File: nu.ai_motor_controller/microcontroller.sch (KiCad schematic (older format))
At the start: 31 parts

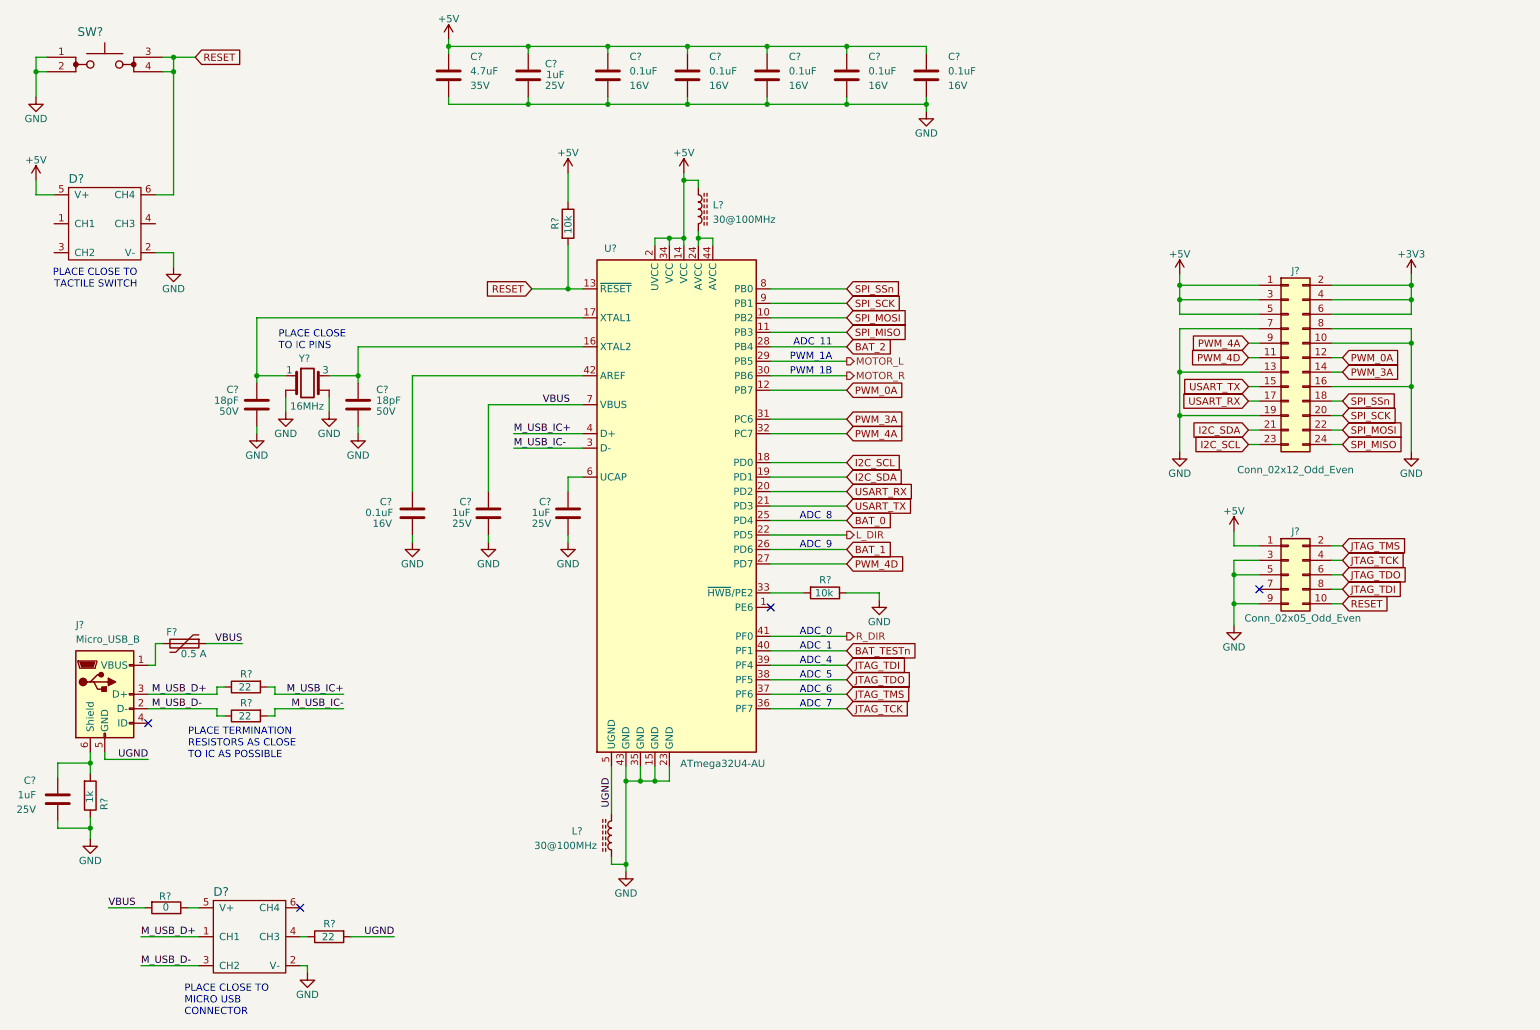
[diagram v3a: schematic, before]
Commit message: automated commit
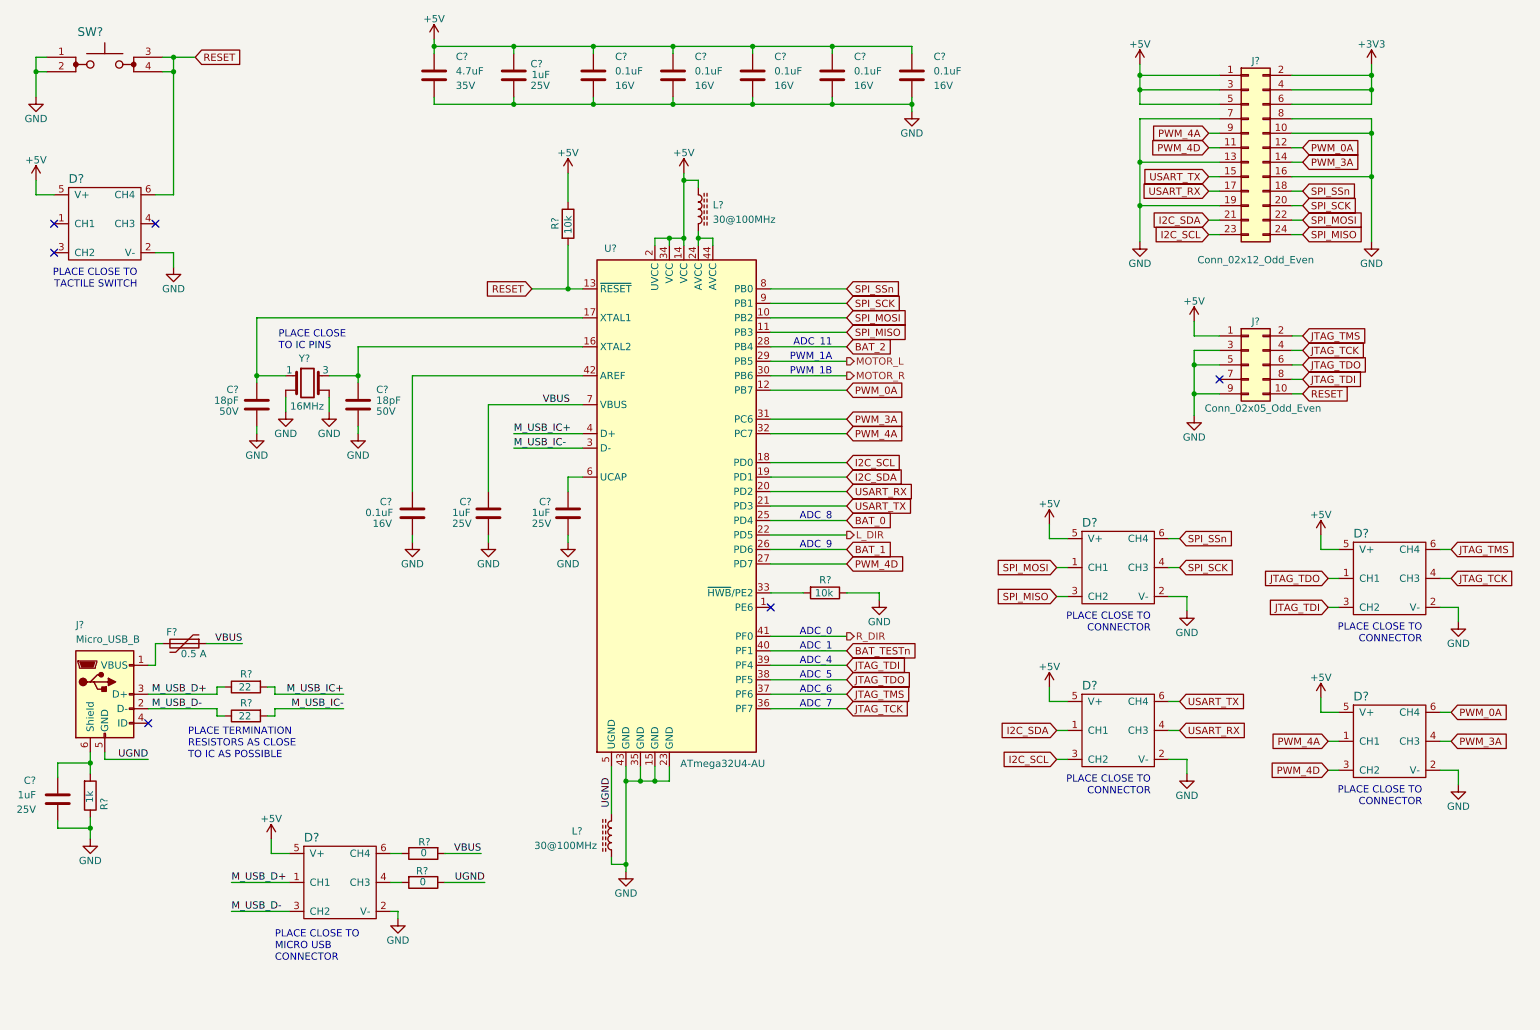
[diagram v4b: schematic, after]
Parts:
- removed R?: RMCF0603FT22R0, 0603, symbol custom:RMCF0603FT22R0
- added D? (x4): CM1293A-04SO, SOT-457, symbol custom:CM1293A-04SO
- added R?: RC0603JR-070RL, Resistor_SMD:R_0603_1608Metric, symbol custom:RC0603JR-070RL
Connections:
- net +5V: now also D?.5 (V+), D?.5 (V+), D?.5 (V+), D?.5 (V+), D?.5 (V+)
- net GND: now also D?.2 (V-), D?.2 (V-), D?.2 (V-), D?.2 (V-)
- net I2C_SCL: now also D?.3 (CH2)
- net I2C_SDA: now also D?.1 (CH1)
- net JTAG_TCK: now also D?.4 (CH3)
- net JTAG_TDI: now also D?.3 (CH2)
- net JTAG_TDO: now also D?.1 (CH1)
- net JTAG_TMS: now also D?.6 (CH4)
- net PWM_0A: now also D?.6 (CH4)
- net PWM_3A: now also D?.4 (CH3)
- net PWM_4A: now also D?.1 (CH1)
- net PWM_4D: now also D?.3 (CH2)
- net SPI_MISO: now also D?.3 (CH2)
- net SPI_MOSI: now also D?.1 (CH1)
- net SPI_SCK: now also D?.4 (CH3)
- net SPI_SSn: now also D?.6 (CH4)
- net UGND: now also R?.1
- net USART_RX: now also D?.4 (CH3)
- net USART_TX: now also D?.6 (CH4)
- net at D?.4 (CH3): now also R?.2
- net at R?.1: now also D?.6 (CH4); no longer D?.5 (V+)
- no-connect marks 4 -> 6
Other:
- note added: "PLACE CLOSE TO\nCONNECTOR"
- moved on the sheet: C?, D?, J?, R?

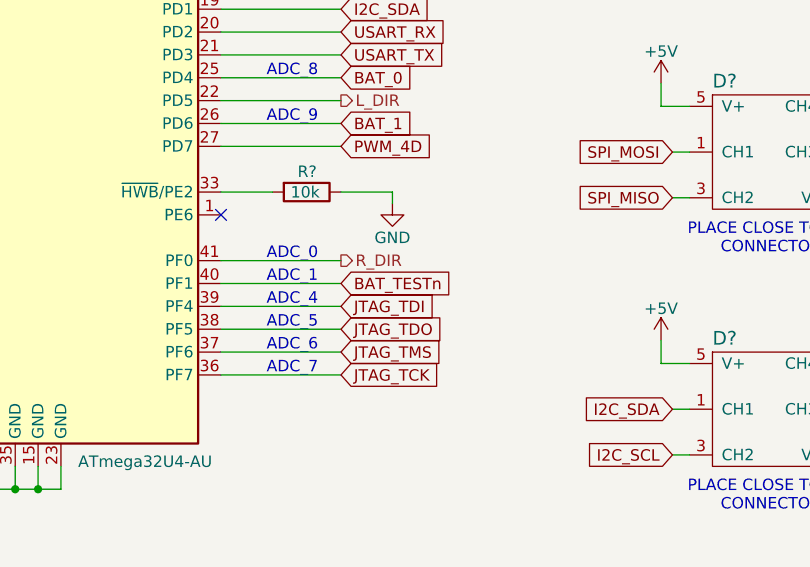
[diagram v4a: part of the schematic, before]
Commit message: automated commit
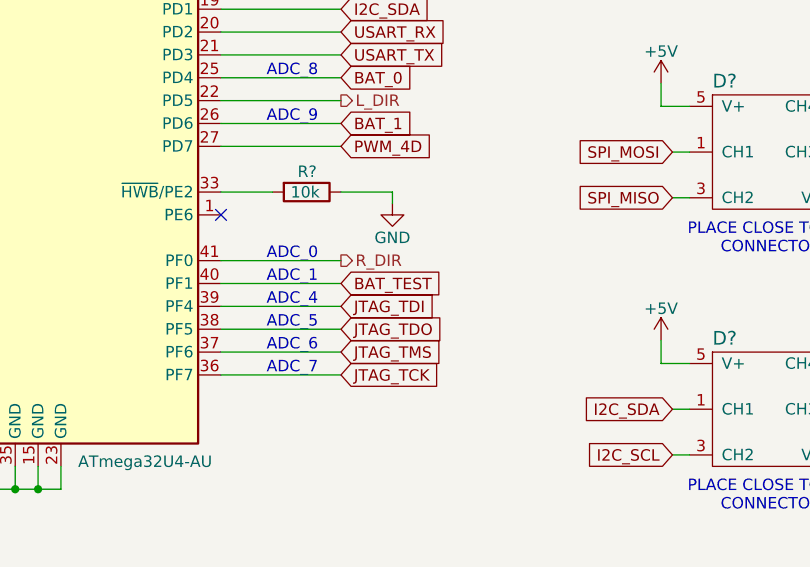
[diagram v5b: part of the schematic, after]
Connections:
- net BAT_TESTn renamed BAT_TEST
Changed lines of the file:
@@
 PWM_4D
 Text GLabel 6375 4950 2    50   Input ~ 0
-BAT_TESTn
+BAT_TEST
 Text GLabel 6375 5050 2    50   Input ~ 0
 JTAG_TDI
